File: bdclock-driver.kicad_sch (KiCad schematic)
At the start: 34 parts, among them J1 PWR, J2 Ctrl, J3 Kathodes, J4 Anodes A, J5 Anodes B, J6 Anodes C, U1 NE555P, U2 LM7805_TO220, U3 74HC4017, U4 74HC595, U5 74HC595, U6 74HC595, U7 74LS138, U8 74LS138

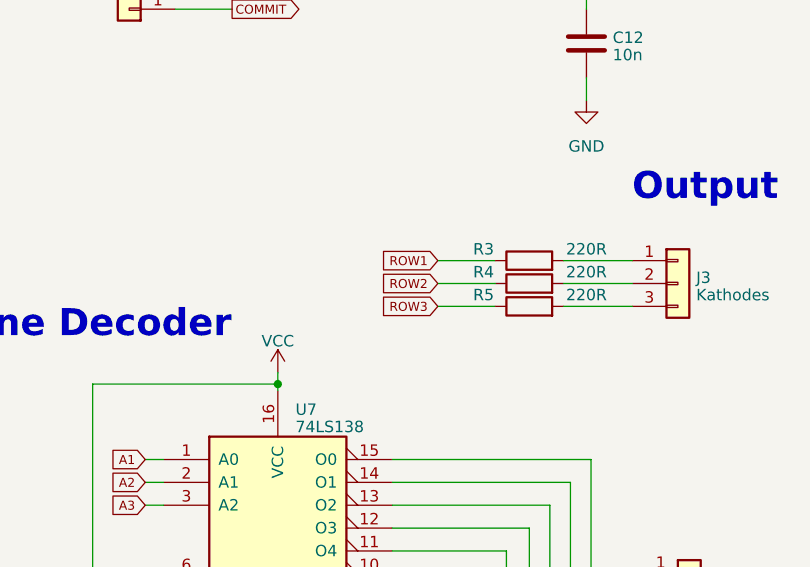
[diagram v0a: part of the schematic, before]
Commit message: :hammer: Improve PCB layout
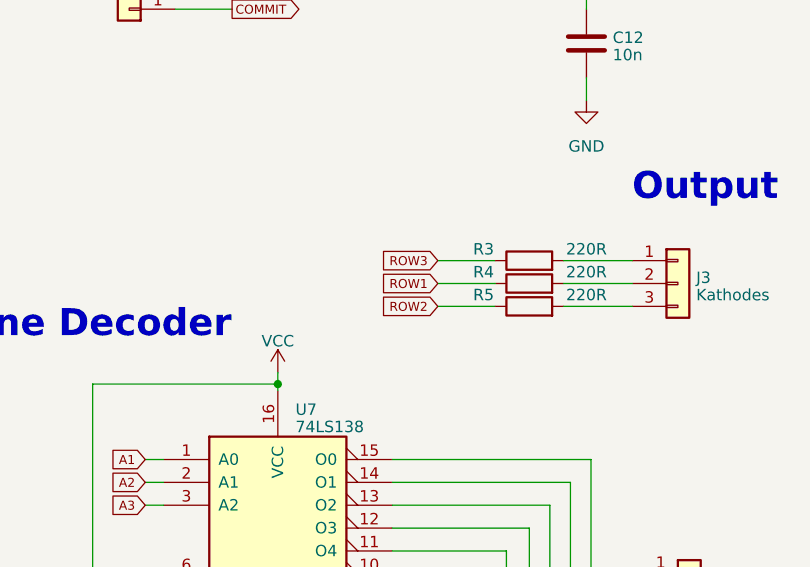
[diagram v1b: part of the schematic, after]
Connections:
- net ROW1: now also R4.1; no longer R3.1
- net ROW2: now also R5.1; no longer R4.1
- net ROW3: now also R3.1; no longer R5.1

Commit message: :art: Finalize the PCB layout
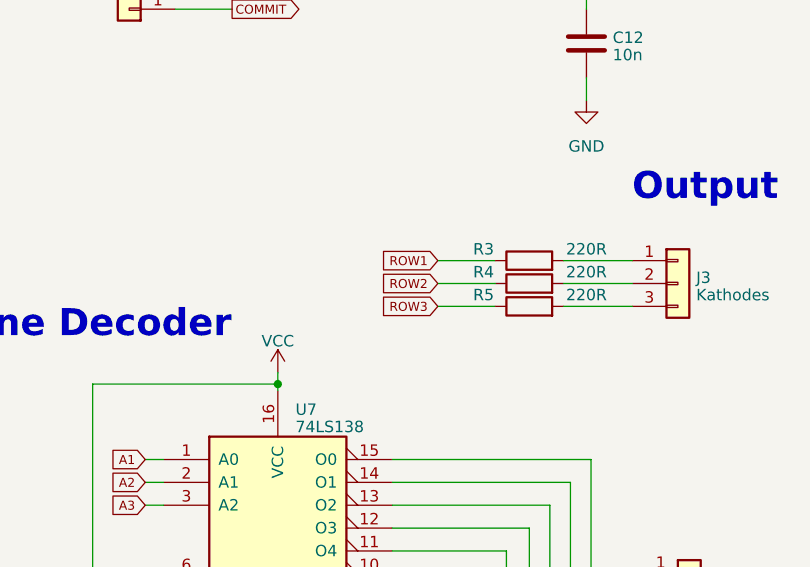
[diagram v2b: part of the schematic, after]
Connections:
- net ROW1: now also R3.1; no longer R4.1
- net ROW2: now also R4.1; no longer R5.1
- net ROW3: now also R5.1; no longer R3.1
